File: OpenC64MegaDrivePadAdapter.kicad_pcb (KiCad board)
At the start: 2 copper layers, 47.8 x 31 mm, 17 parts, among them J1 CONN_01X02, J10 DB9_F_TO_C64, J2 CONN_02X03, J20 DB9_M_TO_PAD, J3 CONN_02X03, J4 CONN_C64_AMI, J99 OSHW_LOGO, Q1 BC547

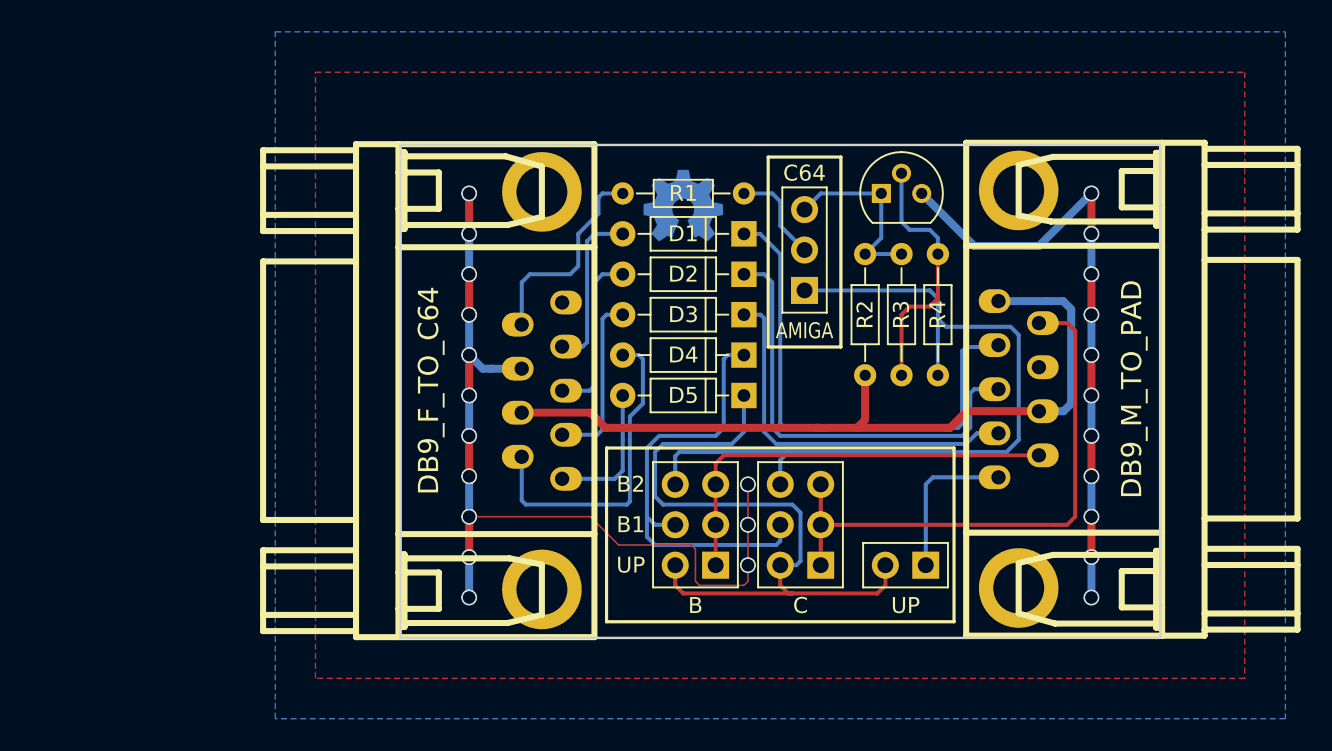
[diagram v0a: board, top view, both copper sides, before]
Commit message: V4 PCB
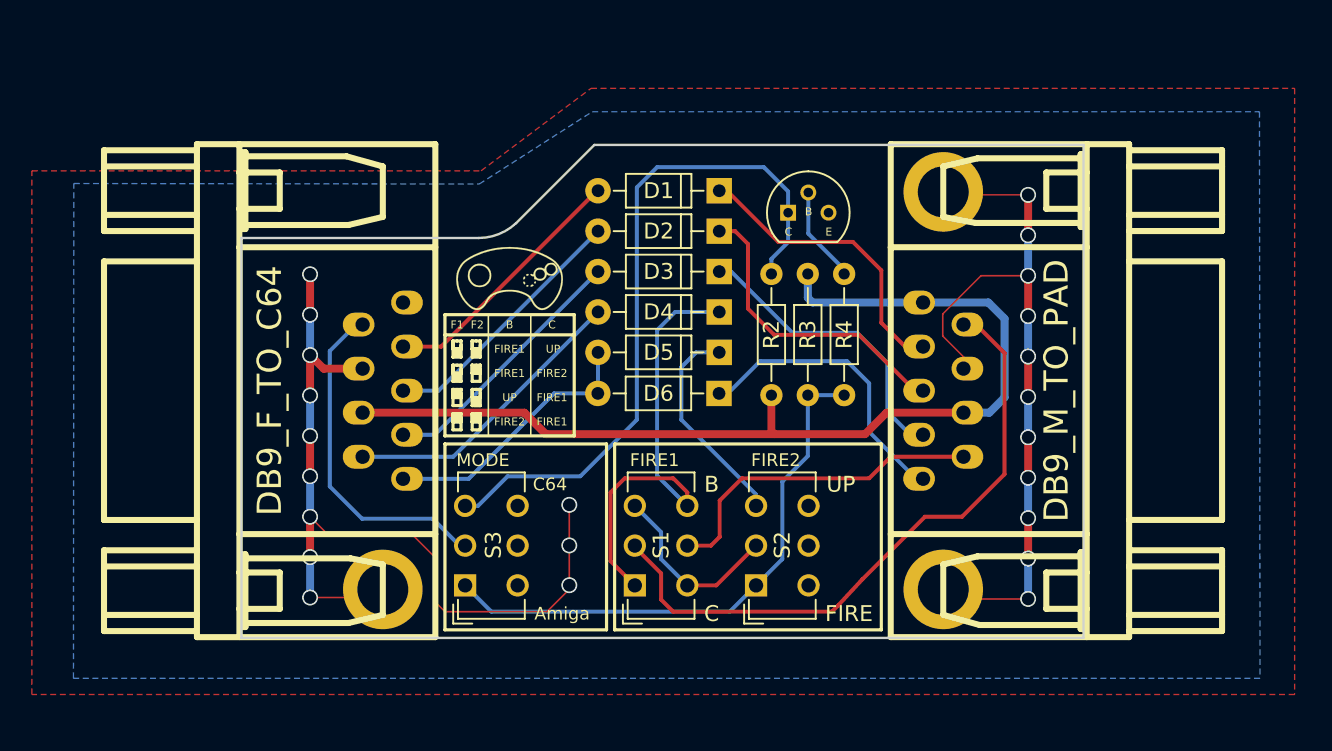
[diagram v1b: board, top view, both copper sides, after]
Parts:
- removed J1: CONN_01X02, Pin_Header_Straight_1x02-ModSilkS
- removed J2, J3: CONN_02X03, OpenC64MegaDrivePadAdapter:Pin_Header_Straight_2x03-ModSilkS
- removed J4: CONN_C64_AMI, Pin_Header_Straight_1x03-ModSilkS
- removed J99: OSHW_LOGO, Symbol_copper_OSHW_6x6mm
- removed R1: 100, Resistors_THT:R_Axial_DIN0204_L3.6mm_D1.6mm_P7.62mm_Horizontal
- added D6: 1N4148, Diodes_THT:D_DO-35_SOD27_P7.62mm_Horizontal, F.Cu at (165.1, 104.0)
- added G***: LOGO, oshw:LOGO, B.Cu at (151.8, 100.5)
- added G***: LOGO, mdpad:LOGO, F.Cu at (151.9, 96.8)
- added S1: JS202011CQN, Buttons_Switches_THT:SW_CuK_JS202011CQN_DPDT_Straight, F.Cu at (159.8, 116.1)
- added S2: JS202011CQN, Buttons_Switches_THT:SW_CuK_JS202011CQN_DPDT_Straight, F.Cu at (167.4, 116.1)
- added S3: JS202011CQN, Buttons_Switches_THT:SW_CuK_JS202011CQN_DPDT_Straight, F.Cu at (149.1, 116.1)
- J10: footprint w_conn_d-sub:DB_9F -> db9:DB_9F
- R3: value 100k -> 10k
- R4: value 2.2k -> 100k
- moved J10 10.0 mm to (136.8, 103.8)
- moved R2 6.02 mm to (168.4, 104.1)
- moved R3 6.02 mm to (170.6, 104.1)
- moved R4 6.02 mm to (172.9, 104.1)
- moved Q1 5.98 mm to (169.4, 92.7)
- moved J20 4.74 mm to (186.3, 103.8)
- moved D1 3.12 mm to (165.1, 91.3)
- moved D3 3.12 mm to (165.1, 96.3)
- moved D2 3.12 mm to (165.1, 93.8)
- moved D4 3.12 mm to (165.1, 98.9)
- moved D5 3.12 mm to (165.1, 101.4)
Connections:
- J10 pad : (no net) -> GND
- J10 pad 5: (no net) -> /pot_y
- J10 pad 8: /gnd -> GND
- J20 pad : (no net) -> GND
- J20 pad 8: /gnd -> GND
- Q1 pad 1: Net-(J4-Pad3) -> Net-(Q1-Pad1)
- Q1 pad 3: /gnd -> GND
- R2 pad 2: Net-(J4-Pad3) -> Net-(Q1-Pad1)
- R3 pad 1: Net-(Q1-Pad2) -> Net-(R3-Pad1)
- R3 pad 2: Net-(J4-Pad3) -> +5V
- R4 pad 1: Net-(J2-Pad6) -> Net-(R3-Pad1)
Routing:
- net GND: track 0.00 -> 101.8 mm, vias 0 -> 23
- net /gnd: track 94.6 -> 0.00 mm, vias 25 -> 0
- net Net-(J2-Pad6): track 51.6 -> 0.00 mm
- net Net-(Q1-Pad1): track 0.00 -> 43.9 mm
- net Net-(R3-Pad1): track 0.00 -> 35.2 mm
- net Net-(D5-Pad1): track 43.6 -> 14.2 mm
- net +5V: track 50.3 -> 63.8 mm
- net /md_right: track 32.1 -> 18.8 mm
- net Net-(J4-Pad3): track 11.8 -> 0.00 mm
- net Net-(S1-Pad3): track 0.00 -> 11.7 mm
- net Net-(Q1-Pad2): track 16.1 -> 6.05 mm
- net /md_left: track 28.1 -> 19.3 mm
- net /md_up: track 9.84 -> 18.5 mm
- net /pot_x: track 13.1 -> 21.7 mm
- net /up: track 8.75 -> 17.1 mm
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- added copper zone on B.Cu, net GND
- added copper zone on F.Cu, net GND
- removed copper zone on B.Cu, net /gnd
- removed copper zone on F.Cu, net /gnd
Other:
- board size 47.8 x 31 mm -> 52.9 x 31 mm
- rule trace_min: 0.2 -> 0.1
- board text added: "Amiga"
- board text added: "E"
- board text added: "F1"
- board text added: "F2"
- board text added: "FIRE"
- board text added: "FIRE1"
- board text added: "FIRE2"
- board text added: "MODE"
- board text added: "V4"
- board text added: "github.com/screwbreaker/ OpenC64MegaDrivePadAdapter"
- board text removed: "AMIGA"
- board text removed: "B1"
- board text removed: "B2"
- board text removed: "V2"
- board text removed: "github.com/SukkoPera/ OpenC64MegaDrivePadAdapter"
